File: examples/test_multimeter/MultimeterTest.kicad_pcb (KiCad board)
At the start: 4 copper layers, 145 x 18 mm, 110 parts, among them sw1 3.9x2.9mm Switch, sw2 3.9x2.9mm Switch

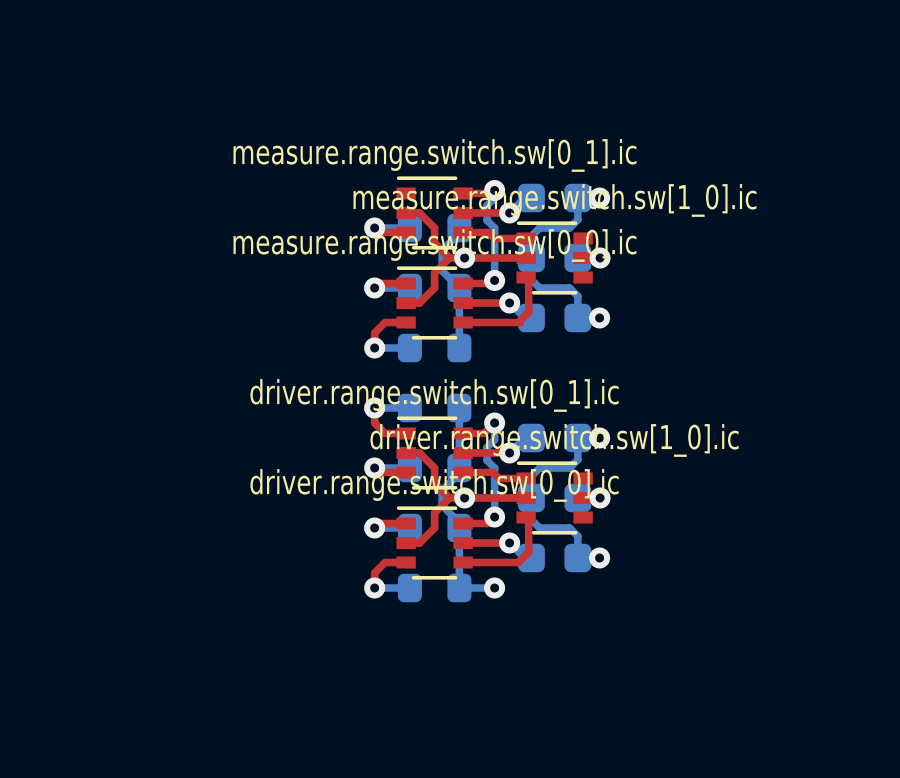
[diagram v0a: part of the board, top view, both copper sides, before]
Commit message: Update MultimeterTest.kicad_pcb
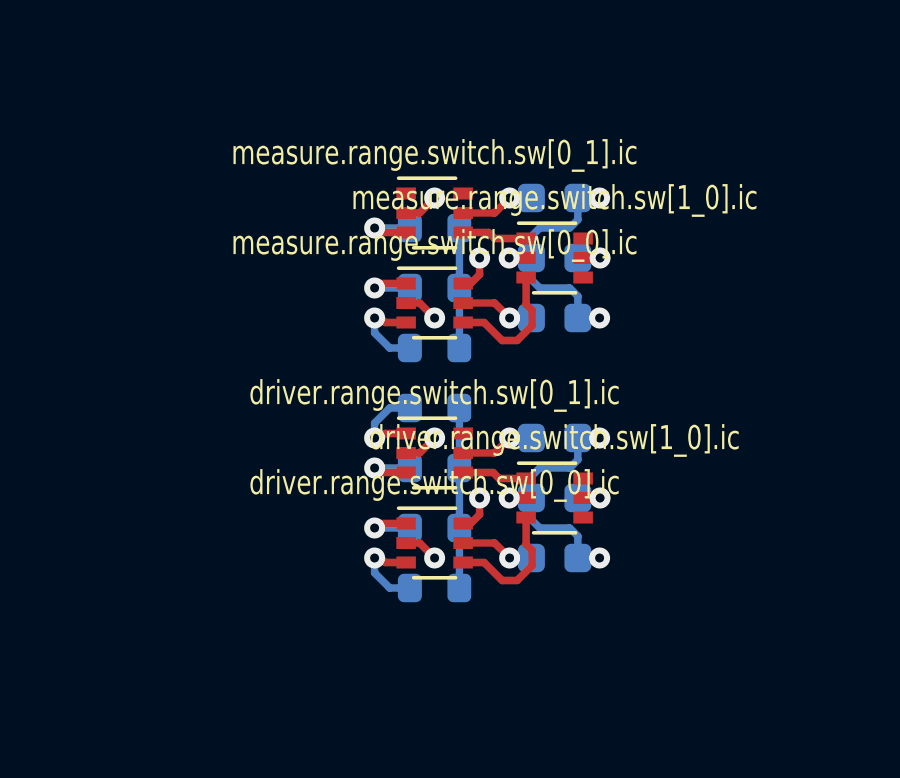
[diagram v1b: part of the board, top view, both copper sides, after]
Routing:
- net gnd: track 67.6 -> 60.3 mm, vias 16 -> 20
- net driver.select.0_0: track 5.68 -> 1.22 mm, vias 2 -> 1
- net mcu.gpio.measure_select_0_0: track 5.39 -> 1.22 mm, vias 2 -> 1
- net vanalog: track 21.6 -> 19.9 mm, vias 8 -> 7
- net driver.range.switch.sw[1_0].inputs.0: track 3.52 -> 4.44 mm
- net measure.range.switch.sw[1_0].inputs.0: track 3.55 -> 4.44 mm
